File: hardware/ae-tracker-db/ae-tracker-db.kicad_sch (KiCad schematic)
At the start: 29 parts, among them J1 Conn_01x04_Plug, J2 Conn_01x01_Pin, J3 Conn_01x04_Socket, J4 Conn_01x16_Pin, U1 SN65HVD231, U2 LIS3DH, U3 BQ25176J, U4 TPS1H000-Q1

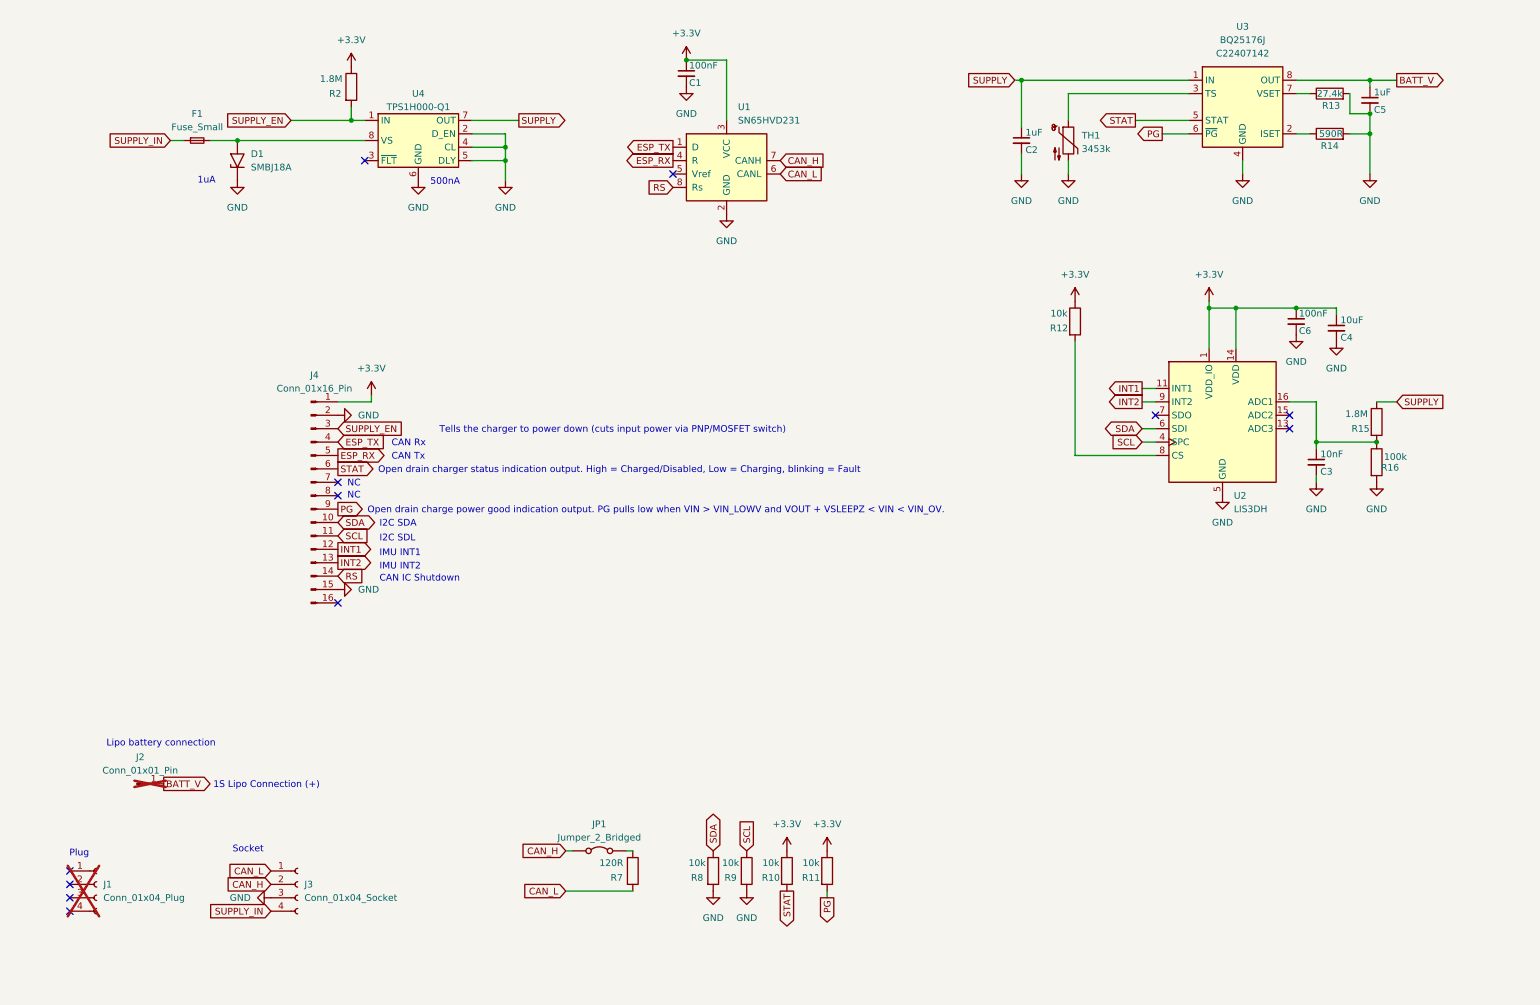
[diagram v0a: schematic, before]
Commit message: v0.0.2 WIP
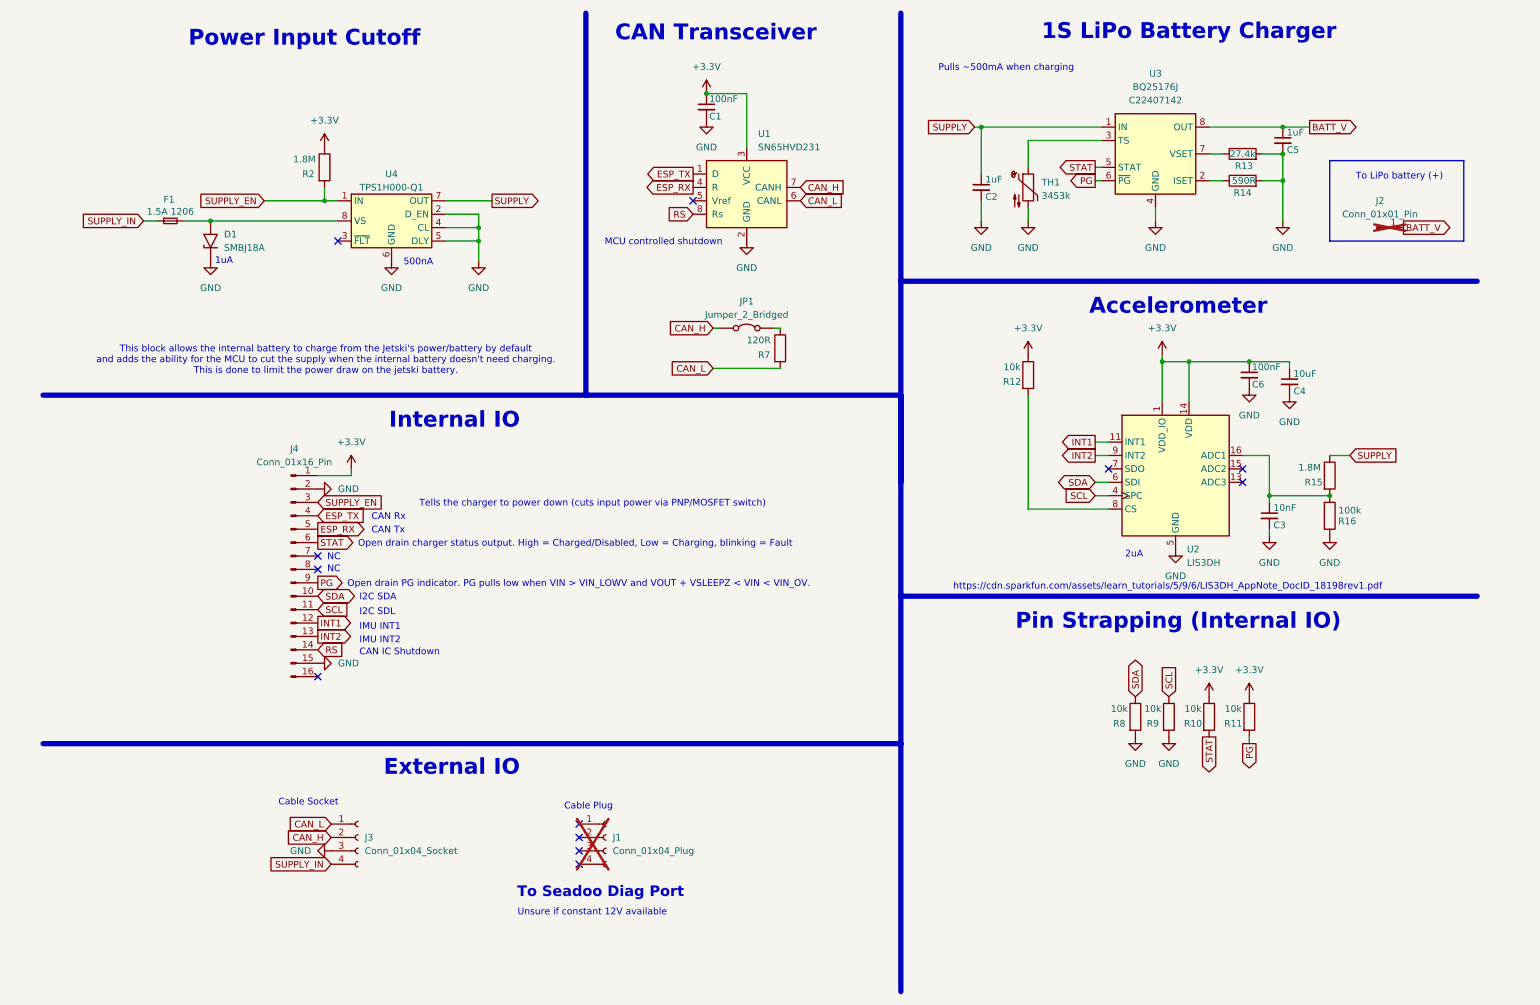
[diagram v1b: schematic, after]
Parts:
- F1: value Fuse_Small -> 1.5A 1206
- J1: footprint (none) -> Connector_PinHeader_2.54mm:PinHeader_1x04_P2.54mm_Vertical
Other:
- note added: "1S LiPo Battery Charger"
- note added: "2uA"
- note added: "Accelerometer"
- note added: "CAN Transceiver"
- note added: "Cable Plug"
- note added: "Cable Socket"
- note added: "External IO"
- note added: "Internal IO"
- note added: "MCU controlled shutdown"
- note added: "Open drain PG indicator. PG pulls low when VIN > VIN_LOWV and VOUT + VSLEEPZ < VIN < VIN_OV."
- note added: "Open drain charger status output. High = Charged/Disabled, Low = Charging, blinking = Fault"
- note added: "Pin Strapping (Internal IO)"
- note added: "Power Input Cutoff"
- note added: "Pulls ~500mA when charging"
- note added: "This block allows the internal battery to charge from the Jetski's power/battery by default and adds the ability for the MCU to cut the supply when the internal battery doesn't need charging. This is done to limit the power draw on the jetski battery."
- note added: "To LiPo battery (+)"
- note added: "To Seadoo Diag Port"
- note added: "Unsure if constant 12V available"
- note added: "https://cdn.sparkfun.com/assets/learn_tutorials/5/9/6/LIS3DH_AppNote_DocID_18198rev1.pdf"
- note removed: "1S Lipo Connection (+)"
- note removed: "Lipo battery connection"
- note removed: "Open drain charge power good indication output. PG pulls low when VIN > VIN_LOWV and VOUT + VSLEEPZ < VIN < VIN_OV."
- note removed: "Open drain charger status indication output. High = Charged/Disabled, Low = Charging, blinking = Fault"
- note removed: "Plug"
- note removed: "Socket"
- moved on the sheet: C1, C2, C3, C4, C5, C6, D1, F1, J1, J2, J3, J4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

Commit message: Fixing wrong part number
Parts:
- J4: LCSC C5370355 -> C2894958
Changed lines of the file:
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@@
 			)
 		)
-		(property "LCSC" "C5370355"
+		(property "LCSC" "C2894958"
 			(at 59.69 118.11 0)
 			(effects
